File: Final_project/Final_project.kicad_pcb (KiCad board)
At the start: 2 copper layers, 54 parts, among them J1 USB4105-GF-A, J2 Conn_01x04, U1 RP2040, U2 MCP1702T-3302E_CB, U3 W25Q128JV, U4 ESP32-WROOM-32, U5 LM393D, Y1 12MHz

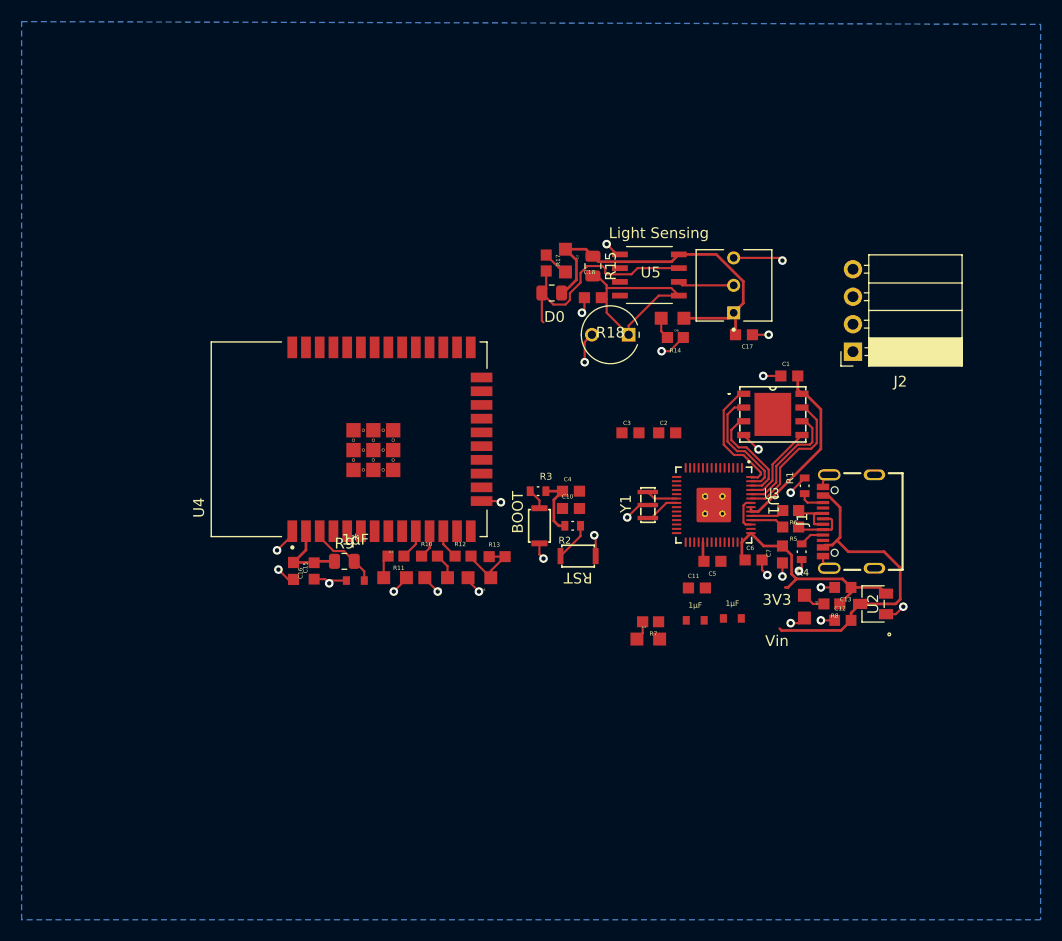
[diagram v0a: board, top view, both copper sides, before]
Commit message: almost finished layout
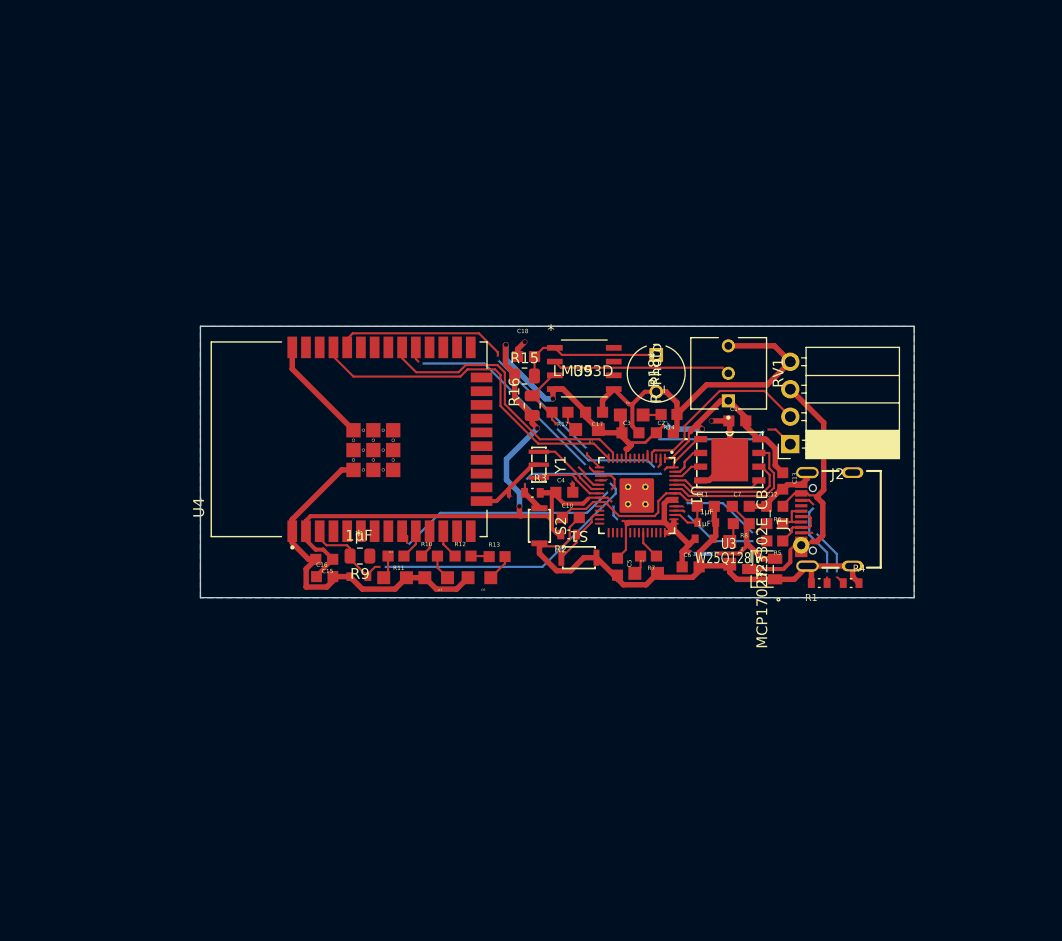
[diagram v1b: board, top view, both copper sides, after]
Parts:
- moved D7 15.8 mm to (126.2, 74.3), turned to 180 degrees
- moved C17 15.6 mm to (126.9, 72.7)
- moved R17 13.9 mm to (123.7, 72.7), turned to 180 degrees
- moved C12 12.3 mm to (143.6, 81.4)
- moved R15 12.0 mm to (120.4, 69.3), turned to 0 degrees
- moved C13 11.3 mm to (144.3, 79.1), turned to -90 degrees
- moved R8 11.2 mm to (140.5, 83.0)
- moved U2 10.7 mm to (142.4, 87.2)
- moved Y1 10.7 mm to (121.8, 77.5)
- moved R16 10.6 mm to (121.1, 72.1), turned to 90 degrees
- moved U5 10.5 mm to (126.0, 68.7), turned to 0 degrees
- moved J2 10.3 mm to (145.0, 75.7)
- moved D6 9.71 mm to (130.3, 73.0), turned to 0 degrees
- moved C9 9.18 mm to (137.3, 82.9)
- moved R1 9.10 mm to (147.7, 88.5), turned to 180 degrees
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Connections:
- R9 pad 1: +3V3 -> +3.3V
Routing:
- net GND: track 53.0 -> 157.4 mm, vias 26 -> 5
- net +3V3: track 87.6 -> 143.9 mm, vias 0 -> 10
- net /GPIO11: track 0.00 -> 32.4 mm
- net /GPIO12: track 0.00 -> 30.2 mm, vias 0 -> 2
- net /GPIO15: track 6.83 -> 35.7 mm, vias 0 -> 2
- net /GPIO10: track 0.00 -> 26.9 mm
- net /GPIO14: track 0.00 -> 25.2 mm, vias 0 -> 2
- net /GPIO13: track 0.00 -> 22.4 mm, vias 0 -> 2
- net /GPIO2: track 0.00 -> 17.4 mm
- net Net-(C10-Pad1): track 3.13 -> 19.8 mm
- net /GPIO3: track 0.00 -> 13.8 mm, vias 0 -> 1
- net Net-(RV1-Pad2): track 5.20 -> 16.5 mm
- net /Light_Sensing/AO: track 21.9 -> 13.7 mm
- net /BOOT: track 13.3 -> 21.2 mm, vias 0 -> 2
- net Net-(U1-Pad55): track 10.9 -> 3.48 mm
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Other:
- board outline added: 66 x 25.1 mm
- board text removed: "3V3"
- board text removed: "D0"
- board text removed: "Light Sensing"
- board text removed: "Vin"
